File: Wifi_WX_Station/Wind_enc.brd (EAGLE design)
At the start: 25.5 x 25.5 mm, 9 parts, among them U1 AS5030

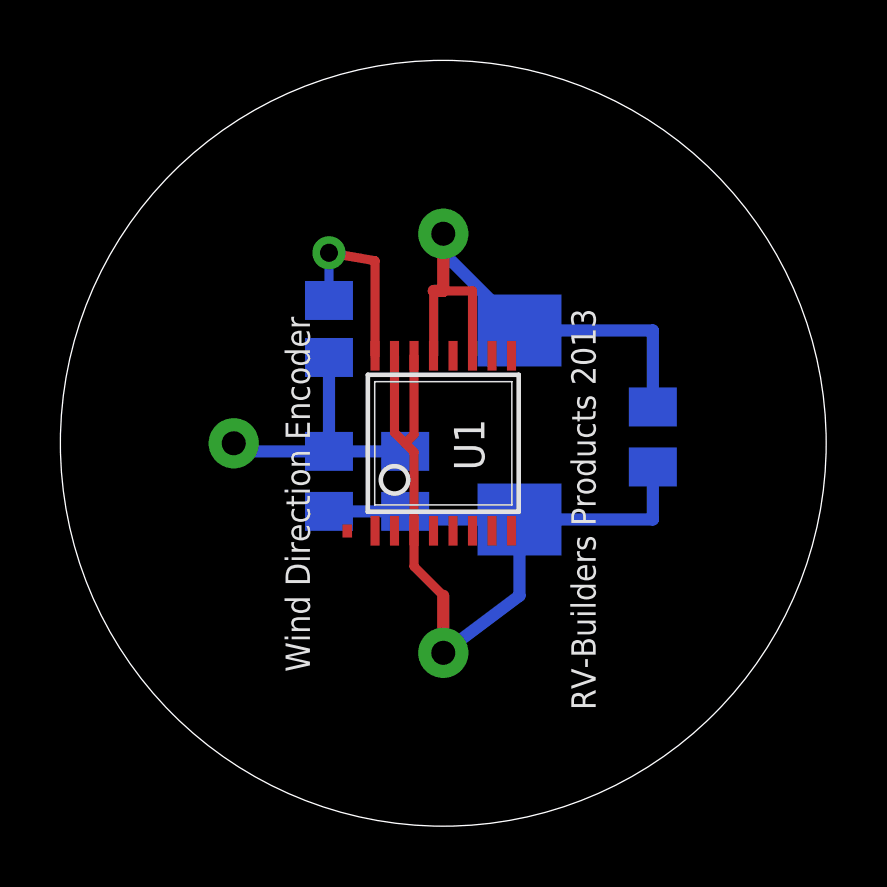
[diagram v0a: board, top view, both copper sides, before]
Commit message: Revision B.1
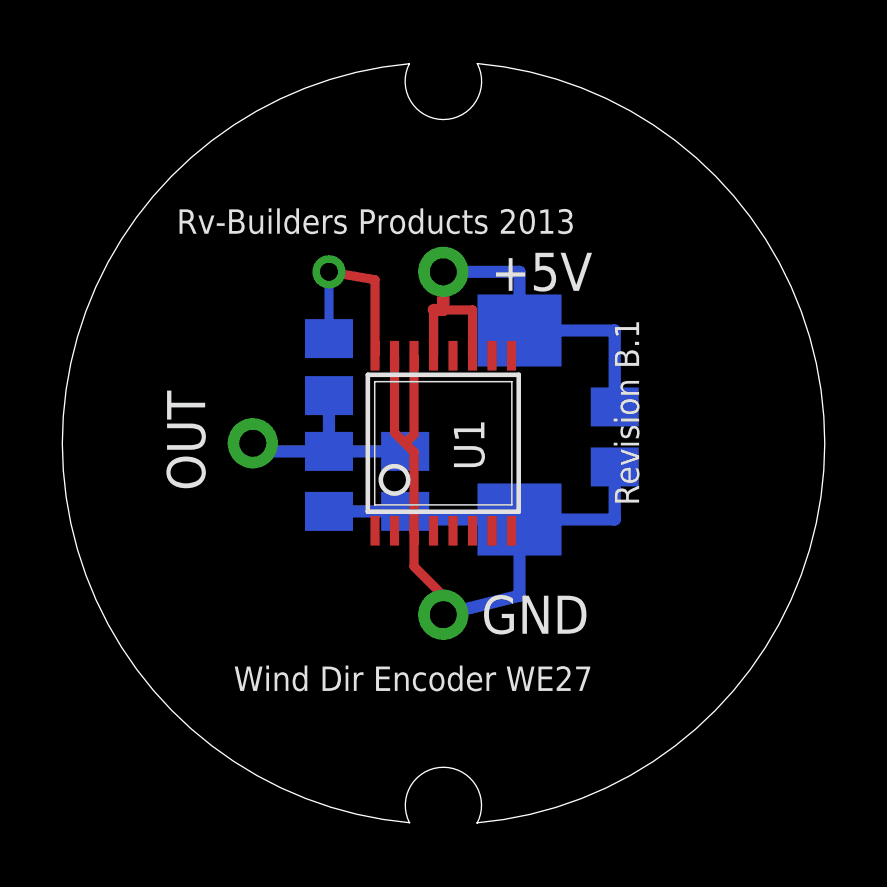
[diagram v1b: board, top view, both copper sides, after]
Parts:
- moved GND 1.27 mm to (14.0, 8.26)
- moved +5V 1.27 mm to (14.0, 19.7)
- moved C1 1.27 mm to (19.7, 14.2)
- moved R6 1.27 mm to (10.2, 16.5)
- moved OUT 0.63 mm to (7.62, 14.0)
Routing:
- net N$1: track 19.1 -> 15.8 mm
- net N$2: track 32.0 -> 28.9 mm
- net N$22: track 8.90 -> 7.21 mm
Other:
- board size 25.5 x 25.5 mm -> 25.4 x 25.3 mm
- board text added: "+5V"
- board text added: "GND"
- board text added: "OUT"
- board text added: "Revision B.1"
- board text added: "Rv-Builders Products 2013"
- board text added: "Wind Dir Encoder WE27"
- board text removed: "."
- board text removed: "RV-Builders Products 2013"
- board text removed: "Wind Direction Encoder"
